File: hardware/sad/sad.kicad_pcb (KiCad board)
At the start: 2 copper layers, 69 parts, among them IC1 LP5012RUKR, J1 USB_C_Receptacle_USB2.0_16P, U1 ATtiny1616-M, U2 MCP73831-2-OT

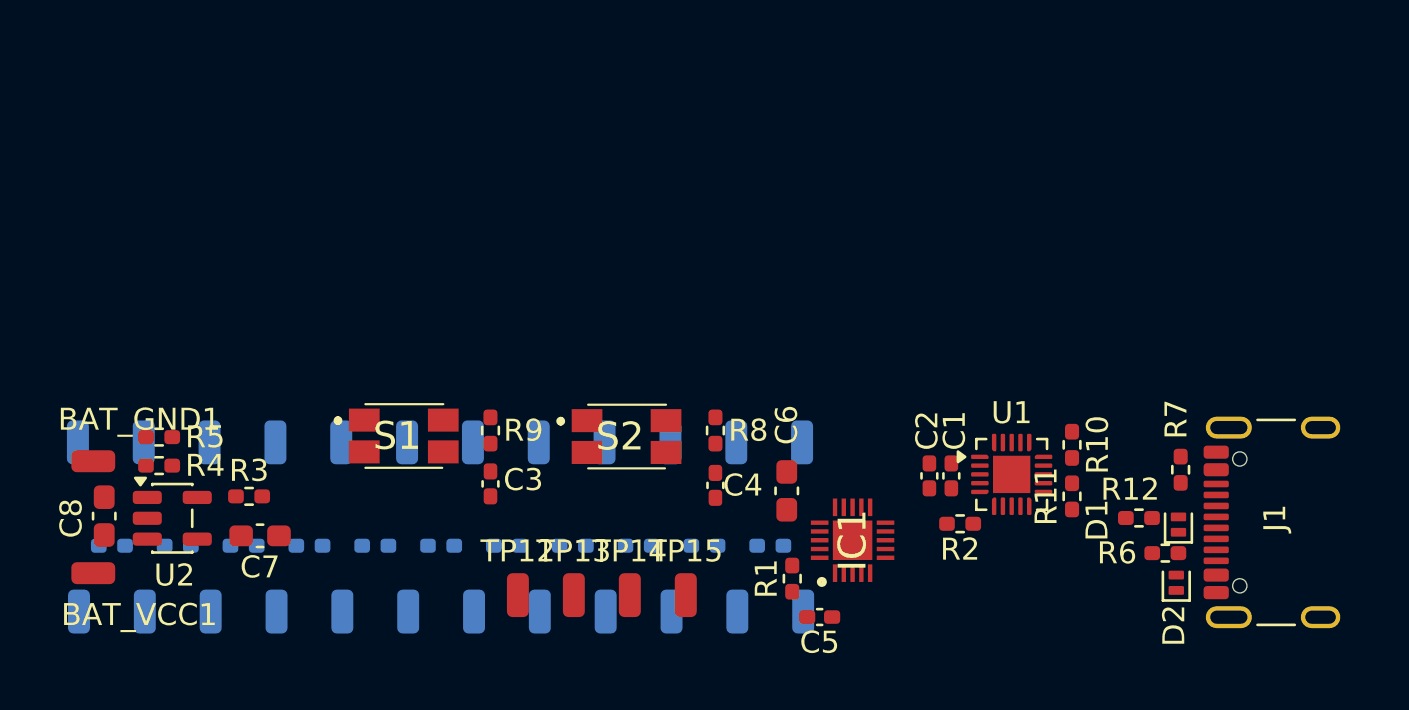
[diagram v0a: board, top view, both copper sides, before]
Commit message: third of the way there
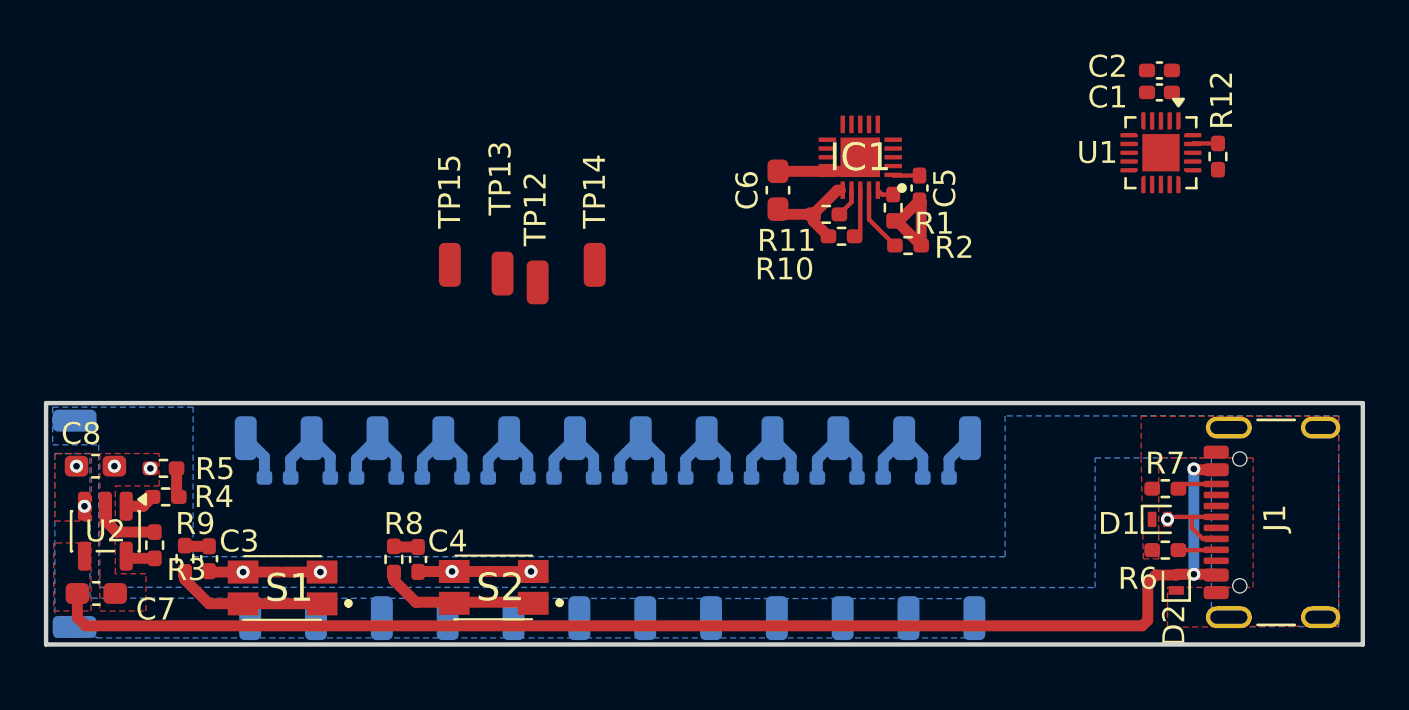
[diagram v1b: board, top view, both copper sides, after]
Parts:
- BAT_GND1, BAT_VCC1: moved to B.Cu
- moved LED_A0 41.6 mm to (169.8, 89.8), turned to 0 degrees
- moved LED_K0 41.4 mm to (169.6, 81.6), turned to 180 degrees
- moved JP0 37.7 mm to (168.0, 83.4)
- moved LED_A1 35.8 mm to (166.8, 89.8), turned to 0 degrees
- moved LED_K1 35.5 mm to (166.6, 81.6), turned to 180 degrees
- moved JP1 31.7 mm to (165.0, 83.4)
- moved LED_A2 29.9 mm to (163.8, 89.8), turned to 0 degrees
- moved LED_K2 29.7 mm to (163.6, 81.6), turned to 180 degrees
- moved LED_K11 26.6 mm to (136.6, 81.6), turned to 180 degrees
- moved LED_A11 26.4 mm to (136.8, 89.8), turned to 0 degrees
- moved JP2 25.7 mm to (162.0, 83.4)
- moved LED_A3 24.2 mm to (160.8, 89.8), turned to 0 degrees
- moved LED_K3 23.9 mm to (160.6, 81.6), turned to 180 degrees
- moved JP10 22.7 mm to (138.0, 83.4)
- moved C2 21.2 mm to (178.2, 64.8), turned to 180 degrees
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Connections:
- U1 pad 1: /SW1 -> unconnected-(U1-PA2-Pad1)
- U1 pad 15: unconnected-(U1-PC0-Pad15) -> /EN
- U1 pad 6: /EN -> /STAT
- U1 pad 7: /SW2 -> /SW1
- U1 pad 8: /STAT -> /SW2
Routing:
- net VBUS: track 0.00 -> 61.0 mm, vias 0 -> 2
- net GND: track 0.00 -> 23.0 mm, vias 0 -> 6
- net Net-(S2-NO_1): track 0.00 -> 7.12 mm
- net Net-(S1-NO_1): track 0.00 -> 7.06 mm
- net VBAT: track 0.00 -> 4.69 mm, vias 0 -> 2
- net Net-(IC1-OUT9): track 0.00 -> 4.35 mm
- net Net-(IC1-OUT8): track 0.00 -> 4.35 mm
- net Net-(IC1-OUT7): track 0.00 -> 4.35 mm
- net Net-(IC1-OUT6): track 0.00 -> 4.35 mm
- net Net-(IC1-OUT5): track 0.00 -> 4.35 mm
- net Net-(IC1-OUT4): track 0.00 -> 4.35 mm
- net Net-(IC1-OUT3): track 0.00 -> 4.35 mm
- net Net-(IC1-OUT2): track 0.00 -> 4.35 mm
- net Net-(IC1-OUT10): track 0.00 -> 4.35 mm
- net Net-(IC1-OUT1): track 0.00 -> 4.35 mm
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- added copper zone on B.Cu, net GND
- added copper zone on F.Cu, net GND
- added copper zone on B.Cu, net VBAT
- added copper zone on F.Cu, net VBAT
- added copper zone on F.Cu, net VBUS
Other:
- board outline added: 60 x 11 mm
